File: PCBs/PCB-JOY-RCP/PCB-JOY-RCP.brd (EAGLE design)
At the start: 30 x 25.9 mm, 23 parts, among them IC1 ADS7828, U2 MIC5205-3.3YM5

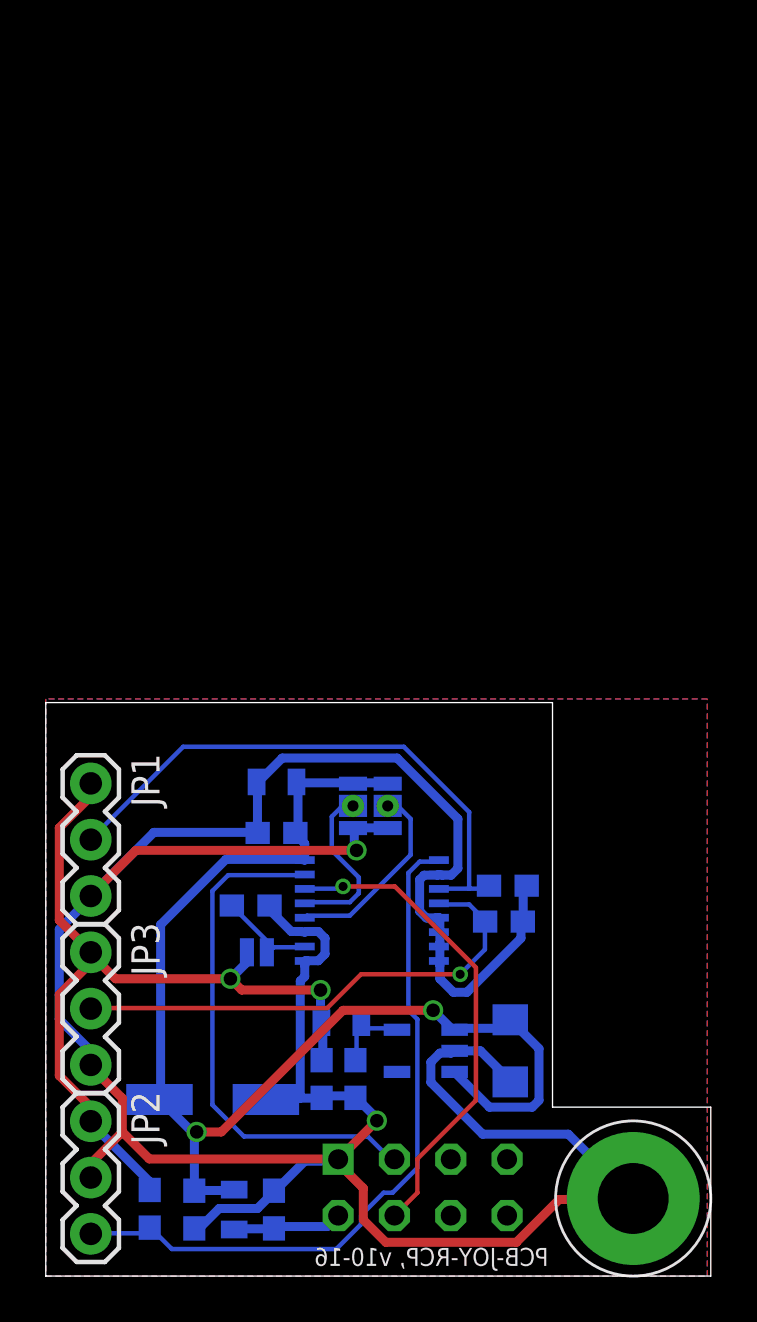
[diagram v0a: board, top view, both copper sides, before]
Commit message: PCB updates
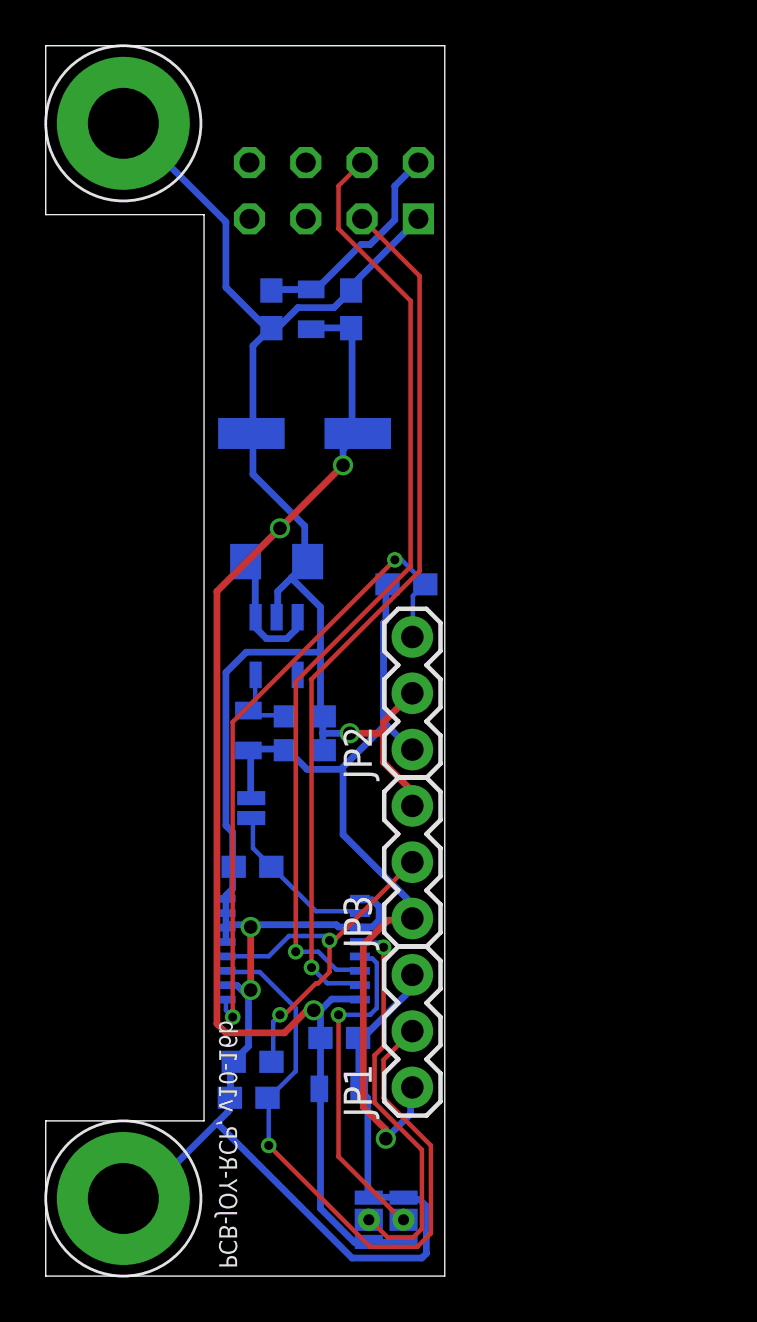
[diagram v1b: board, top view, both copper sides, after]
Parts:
- added U$1: GNDPAD6MM, SKAARHOJ:3.2MMPAD6MM
- moved U$6 53.7 mm to (3.50, 52.0), turned to 180 degrees
- moved SERIAL 45.1 mm to (13.0, 49.0), turned to 90 degrees
- moved C10 41.2 mm to (13.8, 43.6), turned to 90 degrees
- moved L4 40.8 mm to (12.0, 43.6), turned to 270 degrees
- moved C12 40.6 mm to (10.2, 43.6), turned to 270 degrees
- moved R2 30.5 mm to (16.3, 31.2), turned to 180 degrees
- moved PC1 30.3 mm to (11.7, 38.0), turned to 180 degrees
- moved C23 24.5 mm to (10.4, 32.2), turned to 0 degrees
- moved JP2 22.2 mm to (16.5, 23.8), turned to 90 degrees
- moved JP1 20.0 mm to (16.5, 8.51), turned to 90 degrees
- moved U2 19.5 mm to (10.4, 28.4), turned to 180 degrees
- moved U$19 18.8 mm to (16.1, 2.54), turned to 180 degrees
- moved C4 16.5 mm to (11.7, 25.2), turned to 180 degrees
- moved C6 15.1 mm to (9.15, 8.04), turned to 0 degrees
- moved C5 14.8 mm to (11.7, 23.7), turned to 180 degrees
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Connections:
- net GND: now also U$1.P$1
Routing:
- net I2C_SCL: track 22.0 -> 42.8 mm
- net I2C_SDA: track 23.4 -> 39.4 mm, vias 0 -> 1
- net GND: track 139.7 -> 124.1 mm, vias 2 -> 3
- net A0: track 8.91 -> 17.9 mm, vias 0 -> 1
- net 5V: track 56.0 -> 64.7 mm, vias 2 -> 3
- net A1: track 7.81 -> 15.3 mm, vias 0 -> 1
- net JOY_2: track 22.6 -> 17.1 mm, vias 1 -> 2
- net ARD_5V: track 4.93 -> 9.89 mm
- net JOY_1: track 25.8 -> 30.7 mm, vias 0 -> 1
- net FRONT: track 32.1 -> 29.0 mm, vias 0 -> 2
- net REF: track 37.7 -> 40.5 mm, vias 2 -> 1
- net N$1: track 4.85 -> 7.46 mm
- removed copper zone on layer 1, net GND
- removed copper zone on layer 16, net GND
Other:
- board size 30 x 25.9 mm -> 18 x 55.5 mm
- board text added: "PCB-JOY-RCP, v10-16b"
- board text removed: "PCB-JOY-RCP, v10-16"
